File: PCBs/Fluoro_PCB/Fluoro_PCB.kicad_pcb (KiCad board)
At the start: 2 copper layers, 44.5 x 34 mm, 12 parts, among them J1 Conn_02x07_Odd_Even, J2 Conn_02x08_Odd_Even, J3 Conn_02x08_Odd_Even, J4 Conn_01x02_Pin, J5 Conn_01x02_Pin, U1 OPT101P, U3 LM393N

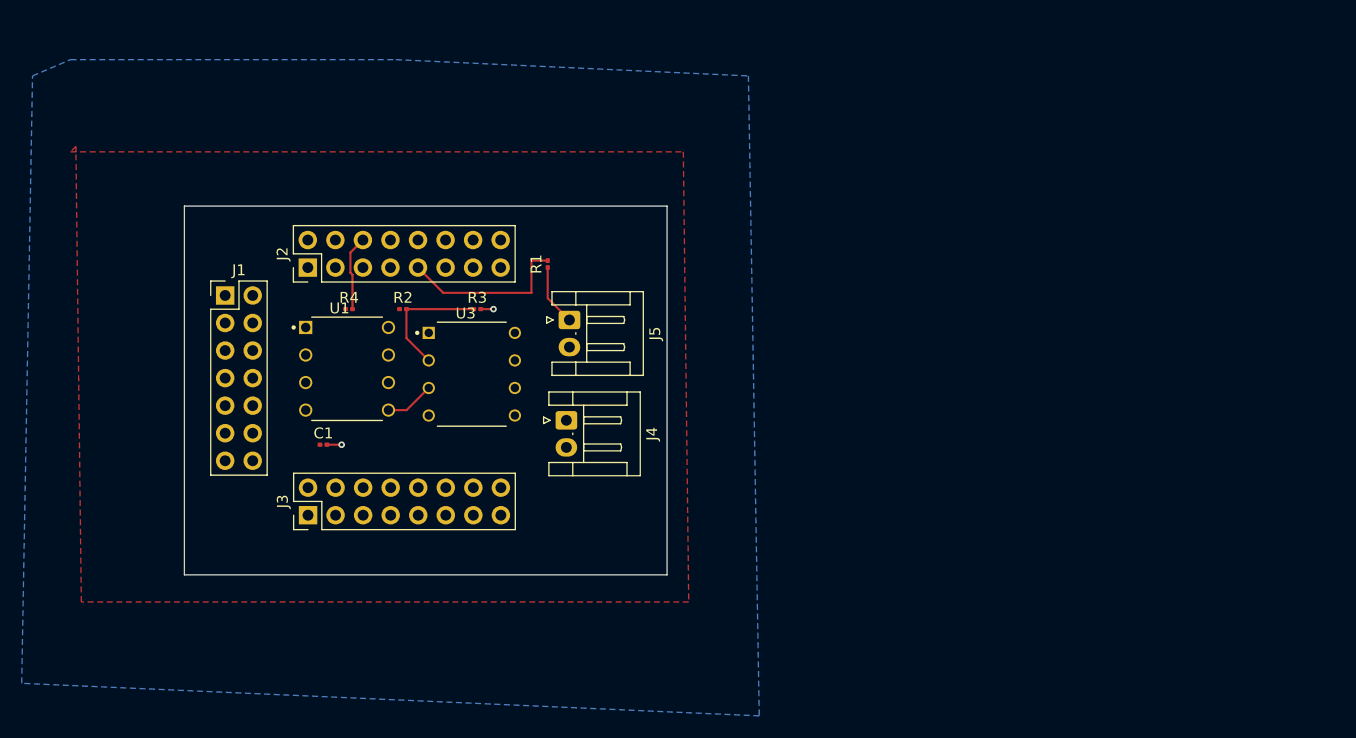
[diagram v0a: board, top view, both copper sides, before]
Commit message: Add files via upload
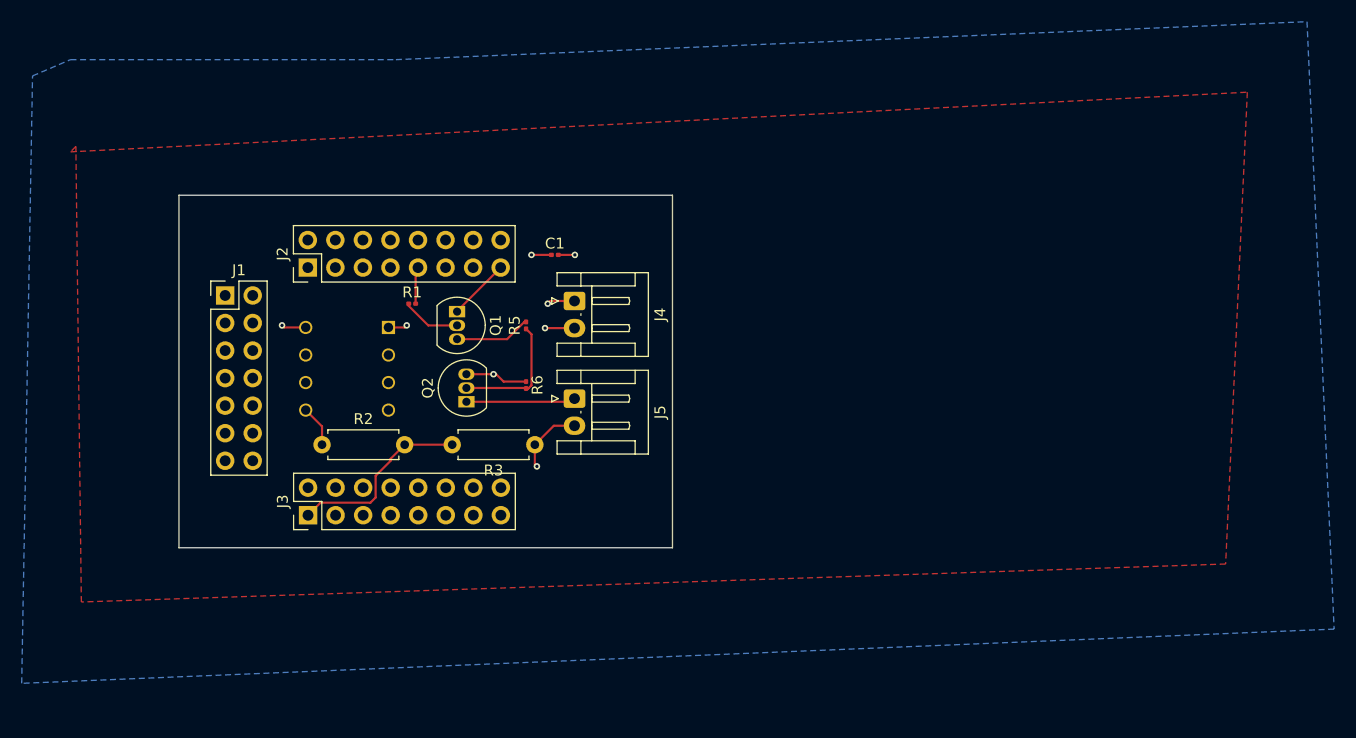
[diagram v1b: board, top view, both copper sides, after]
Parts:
- removed R4: 10000, Resistor_SMD:R_0201_0603Metric
- removed U3: LM393N, LM393N_NOPB:DIP794W45P254L959H508Q8
- added Q1: S8050, Package_TO_SOT_THT:TO-92_Inline, F.Cu at (147.6, 60.7)
- added Q2: S8550, Package_TO_SOT_THT:TO-92_Inline, F.Cu at (148.5, 69.0)
- added R5: 680, Resistor_SMD:R_0201_0603Metric, F.Cu at (154.0, 62.0)
- added R6: 330, Resistor_SMD:R_0201_0603Metric, F.Cu at (154.0, 67.5)
- R2: footprint Resistor_SMD:R_0201_0603Metric -> Resistor_THT:R_Axial_DIN0207_L6.3mm_D2.5mm_P7.62mm_Horizontal
- R3: value 10000 -> 20000; footprint Resistor_SMD:R_0201_0603Metric -> Resistor_THT:R_Axial_DIN0207_L6.3mm_D2.5mm_P7.62mm_Horizontal
- U1: moved to B.Cu
- moved C1 27.6 mm to (156.7, 55.5)
- moved R2 14.6 mm to (135.2, 73.0)
- moved R3 13.6 mm to (154.8, 73.0), turned to 180 degrees
- moved R1 13.0 mm to (143.5, 60.0), turned to 0 degrees
- moved J4 11.0 mm to (158.5, 59.8)
- moved J5 7.27 mm to (158.5, 68.8)
- turned U1 to 180 degrees
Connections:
- J2 pad 1: /6 -> unconnected-(J2-Pin_1-Pad1)
- J3 pad 7: /26 -> unconnected-(J3-Pin_7-Pad7)
- J3 pad 9: /28 -> unconnected-(J3-Pin_9-Pad9)
- R1 pad 1: Net-(J5-Pin_1) -> Net-(Q1-B)
- R2 pad 1: +5V -> Net-(U1-OUTPUT)
- R2 pad 2: Net-(U3-NEG_A) -> /43
- R3 pad 1: Net-(U3-NEG_A) -> GND
- R3 pad 2: GND -> /43
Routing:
- net /43: track 0.00 -> 17.3 mm
- net GND: track 2.54 -> 18.7 mm, vias 2 -> 4
- net /54: track 15.9 -> 3.42 mm
- net +5V: track 0.00 -> 12.0 mm, vias 0 -> 4
- net Net-(U3-NEG_A): track 11.8 -> 0.00 mm
- net Net-(Q2-B): track 0.00 -> 11.6 mm
- net Net-(Q1-C): track 0.00 -> 7.02 mm
- net /59: track 6.93 -> 0.00 mm
- net Net-(Q1-B): track 0.00 -> 5.41 mm
- net Net-(J5-Pin_1): track 5.66 -> 10.1 mm
- net Net-(U1-OUTPUT): track 4.56 -> 3.81 mm
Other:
- board size 44.5 x 34 mm -> 45.5 x 32.5 mm

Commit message: first review
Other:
- board text added: "1) I would not use a plane on top, there is not really a need 2) If something is tht and connects to a plane, it does not need a via 3)Wrong connectors, use jst-GH 4)C1 is just in the middle of nowhere, it should be closer to the power input 5) you have a lot of space, switch smd components to 0805 6) you can bring the jsts on the right closer in, esp when you switch them for the right ones 7) mo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"
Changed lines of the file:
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@@
 		(layer "Edge.Cuts")
+	)
+	(gr_text "1) I would not use a plane on top, there is not really a need\n2) If something is tht and connects to a plane, it does not need a via\n3)Wrong connectors, use jst-GH\n4)C1 is just in the middle of nowhere, it should be closer to the\npower input\n5) you have a lot of space, switch smd components to 0805\n6) you can bring the jsts on the right closer in, esp when you \nswitch them for the right ones\n7) mounting holes + silkscreen pinout\n8) Make sure you double check you can use pin 43 as ADC\n9) add 22nF capactor by the ADC pin"
+		(at 173.69 52.95 0)
+		(layer "User.1")
+		(effects
+			(font
+				(size 1 1)
+				(thickness 0.15)
+			)
+			(justify left bottom)
+		)
 	)
 	(segment

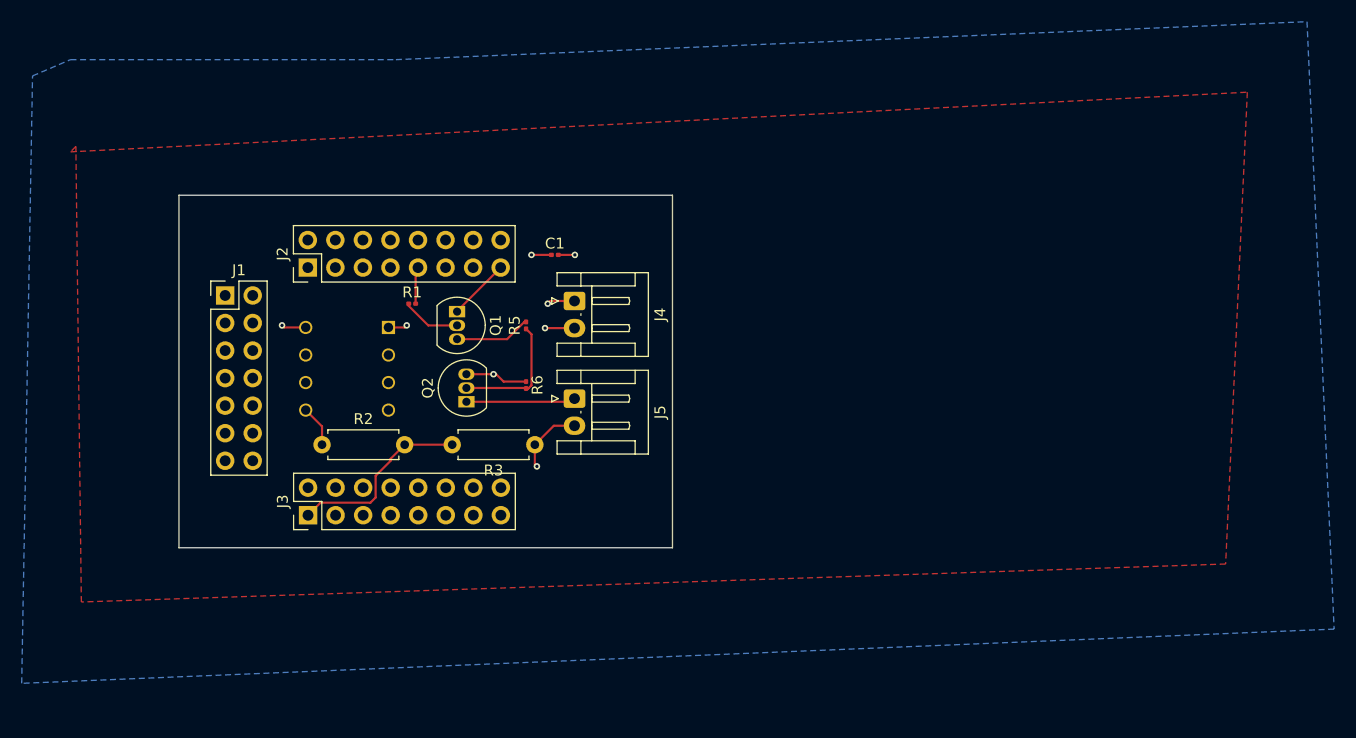
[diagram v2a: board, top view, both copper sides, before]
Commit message: Changes to Fluoro
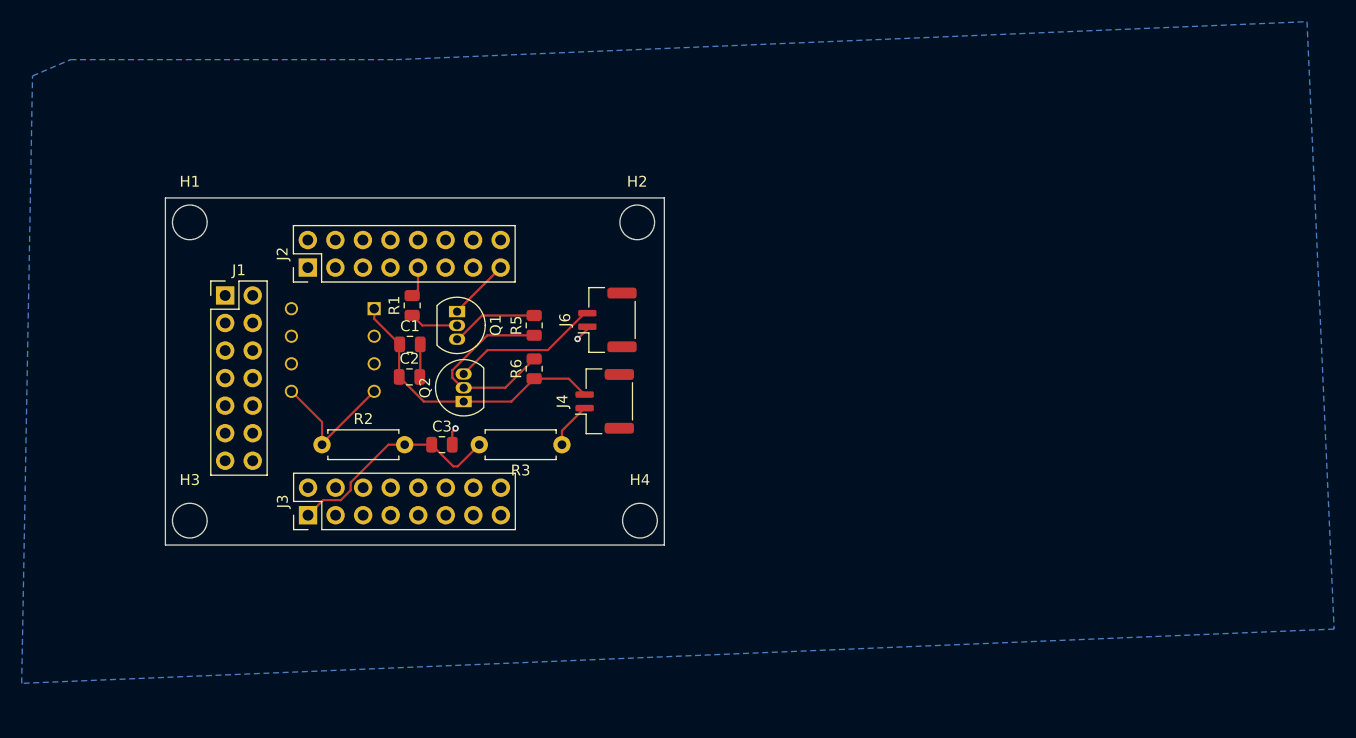
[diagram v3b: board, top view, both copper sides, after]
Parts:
- removed J5: Conn_01x02_Pin, Connector_JST:JST_EH_S2B-EH_1x02_P2.50mm_Horizontal
- added C2: 100nF, Capacitor_SMD:C_0805_2012Metric, F.Cu at (143.2, 66.8)
- added C3: 22uF, Capacitor_SMD:C_0805_2012Metric, F.Cu at (146.2, 73.0)
- added H1: MountingHole, MountingHole:MountingHole_3.2mm_M3_DIN965, F.Cu at (123.0, 52.5)
- added H2: MountingHole, MountingHole:MountingHole_3.2mm_M3_DIN965, F.Cu at (164.2, 52.5)
- added H3: MountingHole, MountingHole:MountingHole_3.2mm_M3_DIN965, F.Cu at (123.0, 80.0)
- added H4: MountingHole, MountingHole:MountingHole_3.2mm_M3_DIN965, F.Cu at (164.5, 80.0)
- added J6: SM02B-GHS-TB, Connector_JST:JST_GH_SM02B-GHS-TB_1x02-1MP_P1.25mm_Horizontal, F.Cu at (161.5, 61.5)
- C1: footprint Capacitor_SMD:C_0201_0603Metric -> Capacitor_SMD:C_0805_2012Metric
- J4: value Conn_01x02_Pin -> SM02B-GHS-TB; footprint Connector_JST:JST_EH_S2B-EH_1x02_P2.50mm_Horizontal -> Connector_JST:JST_GH_SM02B-GHS-TB_1x02-1MP_P1.25mm_Horizontal
- R1, R5, R6: footprint Resistor_SMD:R_0201_0603Metric -> Resistor_SMD:R_0805_2012Metric
- R2: value 10000 -> 18000
- R3: value 20000 -> 22000
- moved C1 15.7 mm to (143.3, 63.8)
- moved J4 9.66 mm to (161.2, 69.0), turned to 90 degrees
- moved R3 2.50 mm to (157.3, 73.0)
- moved U1 2.17 mm to (136.2, 64.3)
- moved R6 1.68 mm to (154.8, 66.0), turned to 90 degrees
- moved R5 0.75 mm to (154.8, 62.0)
- moved Q2 0.25 mm to (148.2, 69.0)
- moved R1 0.16 mm to (143.5, 60.2), turned to 90 degrees
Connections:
- J4 pad 1: +5V -> GND
- J4 pad 2: GND -> +5V
- Q2 pad 1: Net-(J5-Pin_1) -> +5V
- Q2 pad 3: +5V -> Net-(Q2-C)
- R2 pad 1: Net-(U1-OUTPUT) -> Net-(U1-1MOHM_FB)
- U1 pad 4: unconnected-(U1-1MOHM_FB-Pad4) -> Net-(U1-1MOHM_FB)
- U1 pad 5: Net-(U1-OUTPUT) -> Net-(U1-1MOHM_FB)
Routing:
- net +5V: track 12.0 -> 26.8 mm, vias 4 -> 0
- net Net-(Q2-C): track 0.00 -> 13.7 mm
- net Net-(U1-1MOHM_FB): track 0.00 -> 13.0 mm
- net Net-(J5-Pin_1): track 10.1 -> 0.00 mm
- net Net-(Q2-B): track 11.6 -> 18.6 mm
- net Net-(U1-OUTPUT): track 3.81 -> 0.00 mm
- net /43: track 17.3 -> 20.6 mm
- net GND: track 18.7 -> 17.1 mm, vias 4 -> 2
- net Net-(Q1-C): track 7.02 -> 8.01 mm
- net Net-(Q1-B): track 5.41 -> 4.52 mm
- net /54: track 3.42 -> 2.80 mm
- removed copper zone on F.Cu, net +5V
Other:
- board size 45.5 x 32.5 mm -> 46 x 32 mm

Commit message: comments
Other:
- board text added: "You can squisih everything together and make the board smaller, also bring in the left side it doesnt need to be that far out Some pads are not connected to GND, run the DRC what are the current requirements, some traces might need to be thicker if you are expecting higher current Use the schematic to help with placement, if the schematic shows a capcitor near a specific component like a power he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"
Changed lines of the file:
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@@
 		(layer "Edge.Cuts")
+	)
+	(gr_text "You can squisih everything together and make the board smaller, also bring in the left side it \ndoesnt need to be that far out\n\nSome pads are not connected to GND, run the DRC\n\nwhat are the current requirements, some traces might need to \nbe thicker if you are expecting higher current\n\nUse the schematic to help with placement, if the schematic shows a capcitor near\na specific component like a power header, then the capacitor should be\nclose to that. Right now, all the capacitors are just next to each other\nwhich is not really their purpose\n"
+		(at 122.32 39.44 0)
+		(layer "Edge.Cuts")
+		(effects
+			(font
+				(size 1 1)
+				(thickness 0.15)
+			)
+			(justify left bottom)
+		)
 	)
 	(gr_text "1) I would not use a plane on top, there is not really a need\n2) If something is tht and connects to a plane, it does not need a via\n3)Wrong connectors, use jst-GH\n4)C1 is just in the middle of nowhere, it should be closer to the\npower input\n5) you have a lot of space, switch smd components to 0805\n6) you can bring the jsts on the right closer in, esp when you \nswitch them for the right ones\n7) mounting holes + silkscreen pinout\n8) Make sure you double check you can use pin 43 as ADC\n9) add 22nF capactor by the ADC pin"
